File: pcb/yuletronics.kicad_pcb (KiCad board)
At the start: 2 copper layers, 45 x 50 mm, 35 parts, among them IC1 STM32F042F6P6, IC2 MCP1700, IC3 TLV61225, J1 BATT, J2 MICROUSB, P1 SWD_TC, SW1 BOOTLOAD, SW2 PWR_SWITCH

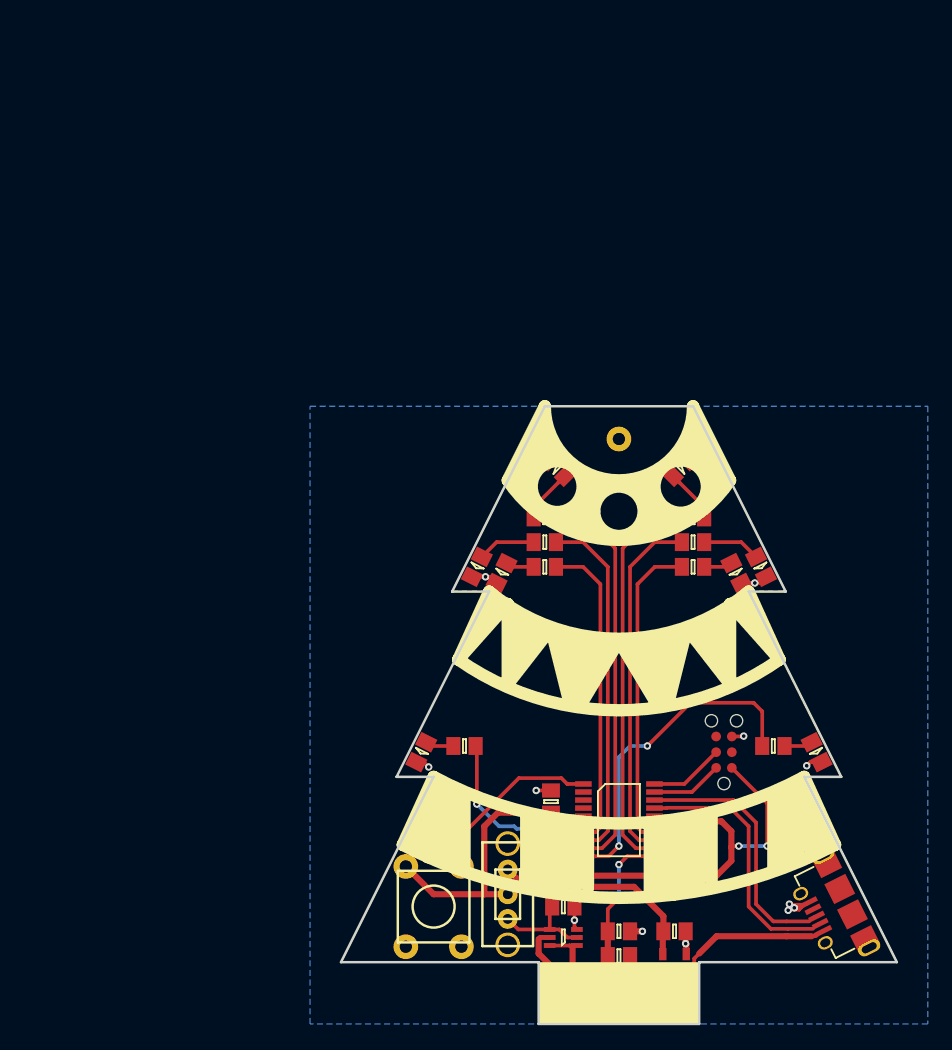
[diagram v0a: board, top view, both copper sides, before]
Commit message: Version 1
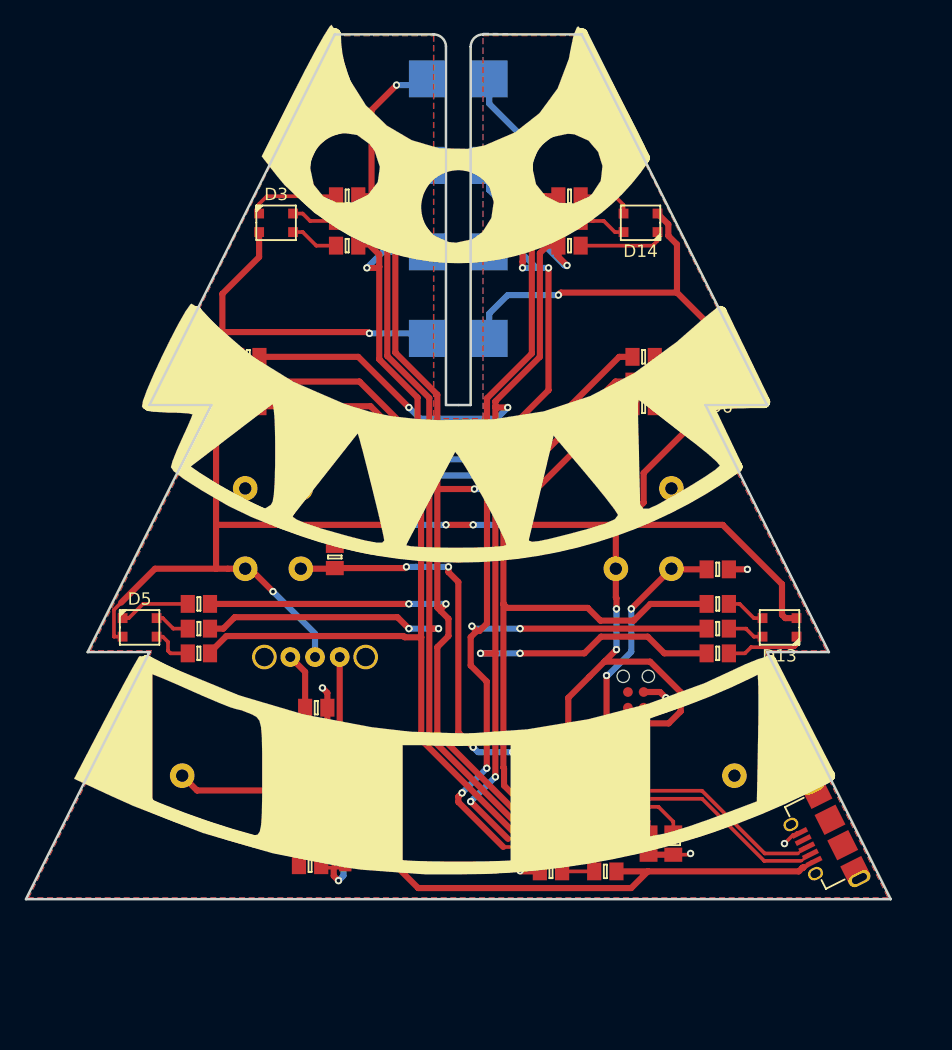
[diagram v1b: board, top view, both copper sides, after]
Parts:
- removed D1, D2, D4, D7, D8: LED, agg:0805-LED
- removed R10, R11, R5, R6, R8, R9: R, agg:0805
- added D10: LED_RABG, yule:CREE_RGB_LED, F.Cu at (95.8, 82.8)
- added D13: LED_RABG, yule:CREE_RGB_LED, F.Cu at (143.0, 102.9)
- added D14: LED_RABG, yule:CREE_RGB_LED, F.Cu at (131.8, 70.2)
- added J3: CONN_01x08, yule:Interboard, B.Cu at (117.0, 55.5)
- added R12: 510, agg:0805, F.Cu at (108.0, 70.0)
- added R15: 510, agg:0805, F.Cu at (108.0, 72.0)
- added R17: 510, agg:0805, F.Cu at (96.0, 101.0)
- added R18: 510, agg:0805, F.Cu at (132.0, 85.0)
- added R20: 510, agg:0805, F.Cu at (96.0, 103.0)
- added R21: 510, agg:0805, F.Cu at (132.0, 83.0)
- added R23: 510, agg:0805, F.Cu at (96.0, 105.0)
- added R24: 510, agg:0805, F.Cu at (132.0, 81.0)
- added R26: 510, agg:0805, F.Cu at (100.0, 81.0)
- added R29: 510, agg:0805, F.Cu at (100.0, 83.0)
- added R32: 510, agg:0805, F.Cu at (100.0, 85.0)
- added R35: 510, agg:0805, F.Cu at (138.0, 105.0)
- added R36: 510, agg:0805, F.Cu at (126.0, 72.0)
- added R38: 510, agg:0805, F.Cu at (138.0, 103.0)
- added R39: 510, agg:0805, F.Cu at (126.0, 70.0)
- added R41: 510, agg:0805, F.Cu at (138.0, 101.0)
- added R42: 510, agg:0805, F.Cu at (126.0, 68.0)
- added SW3: BUTTON, yule:MOM_SWITCH, B.Cu at (132.0, 94.9)
- added X1: Silk_art, yule:tree_silk_scaled, F.Cu at (117.0, 89.8)
- D3, D5, D6: value LED -> LED_RABG; footprint agg:0805-LED -> yule:CREE_RGB_LED
- R4: value R -> 10k
- R7: value R -> 510
- SW1: footprint agg:MOM_SWITCH -> yule:MOM_SWITCH; moved to B.Cu
- SW2: moved to B.Cu
- moved D5 55.7 mm to (91.2, 102.9), turned to 0 degrees
- moved SW1 33.2 mm to (102.0, 94.9), turned to 270 degrees
- moved C5 32.6 mm to (105.0, 119.6), turned to 180 degrees
- moved D3 32.2 mm to (102.2, 70.2), turned to 0 degrees
- moved R7 30.5 mm to (108.0, 68.0), turned to 0 degrees
- moved C6 30.0 mm to (105.0, 122.2), turned to 180 degrees
- moved IC2 27.1 mm to (109.0, 121.4), turned to 0 degrees
- moved L1 25.8 mm to (105.5, 114.7)
- moved C7 25.7 mm to (105.5, 109.4)
- moved C4 25.6 mm to (105.5, 117.5)
- moved IC3 25.5 mm to (105.5, 112.2)
- moved R4 25.0 mm to (138.0, 98.2), turned to 0 degrees
- moved SW2 24.7 mm to (105.4, 105.3), turned to 0 degrees
- moved R1 24.2 mm to (107.0, 97.2), turned to 90 degrees
- moved J1 13.9 mm to (117.0, 114.9), turned to 180 degrees
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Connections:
- D3 pad 1: GND -> Net-(D3-Pad1)
- D3 pad 2: Net-(D3-Pad2) -> 3v3
- D5 pad 1: GND -> Net-(D5-Pad1)
- D5 pad 2: Net-(D5-Pad2) -> 3v3
- D6 pad 1: GND -> Net-(D6-Pad1)
- D6 pad 2: Net-(D6-Pad2) -> 3v3
- IC1 pad 10: /LED5 -> /LED2G
- IC1 pad 12: /LED6 -> /LED2B
- IC1 pad 13: /LED7 -> /BUTTON
- IC1 pad 14: /LED8 -> (no net)
- IC1 pad 2: Net-(IC1-Pad2) -> (no net)
- IC1 pad 3: Net-(IC1-Pad3) -> (no net)
- IC1 pad 4: Net-(IC1-Pad4) -> (no net)
- IC1 pad 6: /LED1 -> /LED1R
- IC1 pad 7: /LED2 -> /LED1G
- IC1 pad 8: /LED3 -> /LED1B
- IC1 pad 9: /LED4 -> /LED2R
- J2 pad 4: Net-(J2-Pad4) -> (no net)
- J2 pad S: Net-(J2-PadS) -> (no net)
- P1 pad 3: Net-(P1-Pad3) -> (no net)
- P1 pad 6: Net-(P1-Pad6) -> (no net)
- R4 pad 1: /LED1 -> /BUTTON
- R4 pad 2: Net-(D1-Pad2) -> GND
- R7 pad 1: /LED4 -> Net-(D3-Pad1)
- R7 pad 2: Net-(D4-Pad2) -> /LED1R
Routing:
- net 3v3: track 63.9 -> 226.8 mm, vias 2 -> 14
- net /LED2G: track 0.00 -> 115.4 mm, vias 0 -> 7
- net /LED2R: track 0.00 -> 113.2 mm, vias 0 -> 7
- net /LED1R: track 0.00 -> 110.4 mm, vias 0 -> 5
- net /LED2B: track 0.00 -> 110.3 mm, vias 0 -> 6
- net /LED1G: track 0.00 -> 106.3 mm, vias 0 -> 5
- net /LED1B: track 0.00 -> 103.3 mm, vias 0 -> 3
- net /LED6: track 32.1 -> 0.00 mm
- net /LED4: track 32.1 -> 0.00 mm
- net /LED7: track 28.7 -> 0.00 mm
- net /LED3: track 28.7 -> 0.00 mm
- net /BUTTON: track 0.00 -> 28.7 mm, vias 0 -> 4
- net /LED5: track 26.9 -> 0.00 mm, vias 2 -> 0
- net /LED8: track 25.4 -> 0.00 mm
- net /LED2: track 25.4 -> 0.00 mm
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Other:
- board size 45 x 50 mm -> 70 x 70 mm
- board text added: "Bootload"
- board text added: "Power"
